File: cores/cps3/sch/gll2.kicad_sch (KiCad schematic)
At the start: 1 part

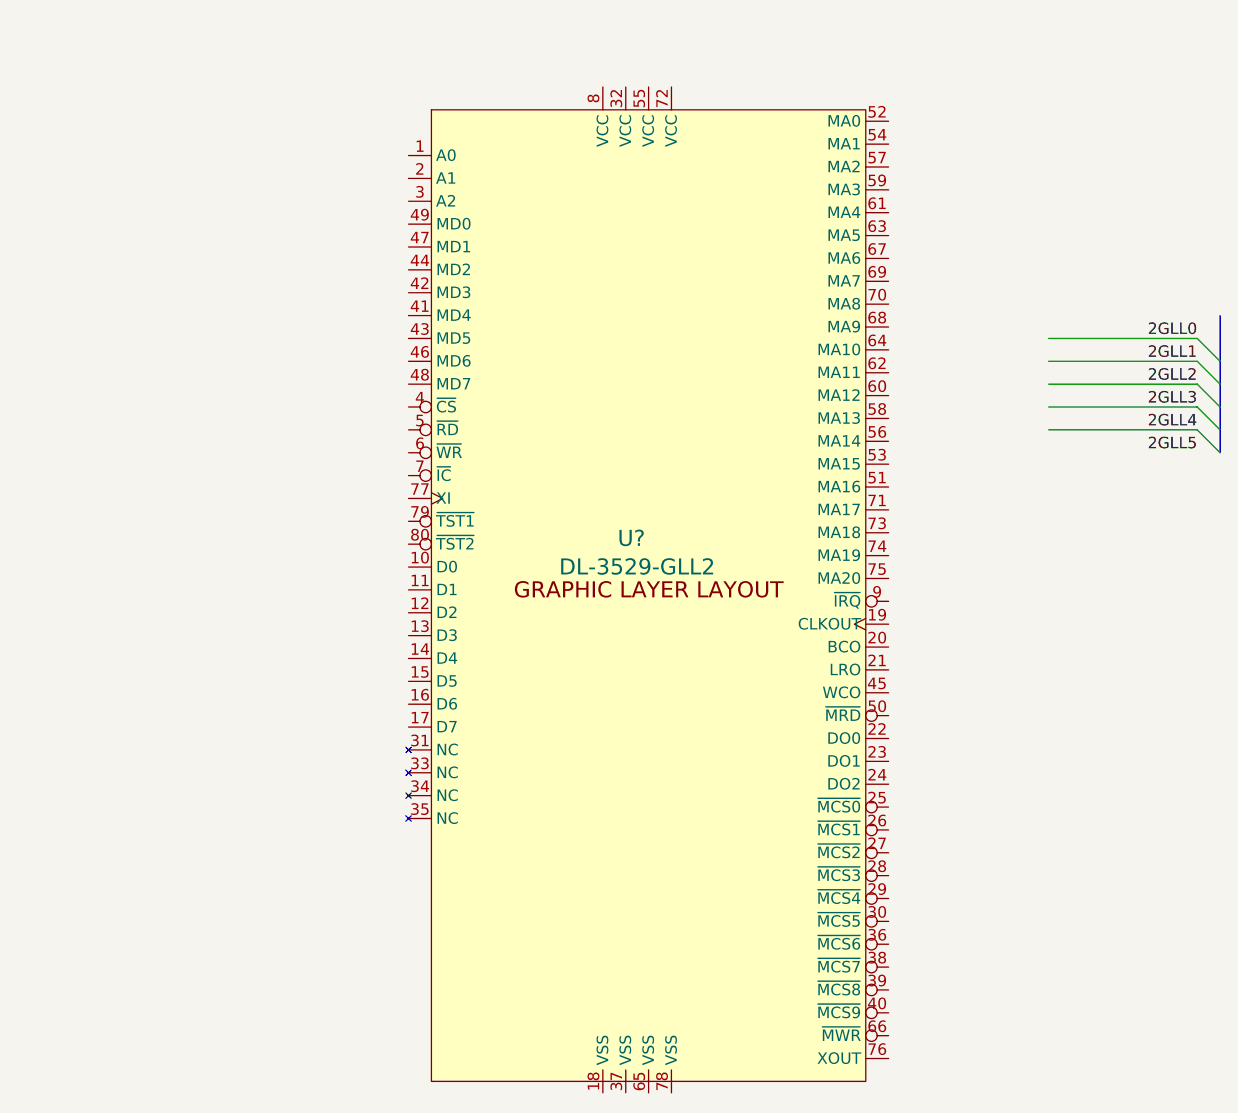
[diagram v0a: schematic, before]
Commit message: iou
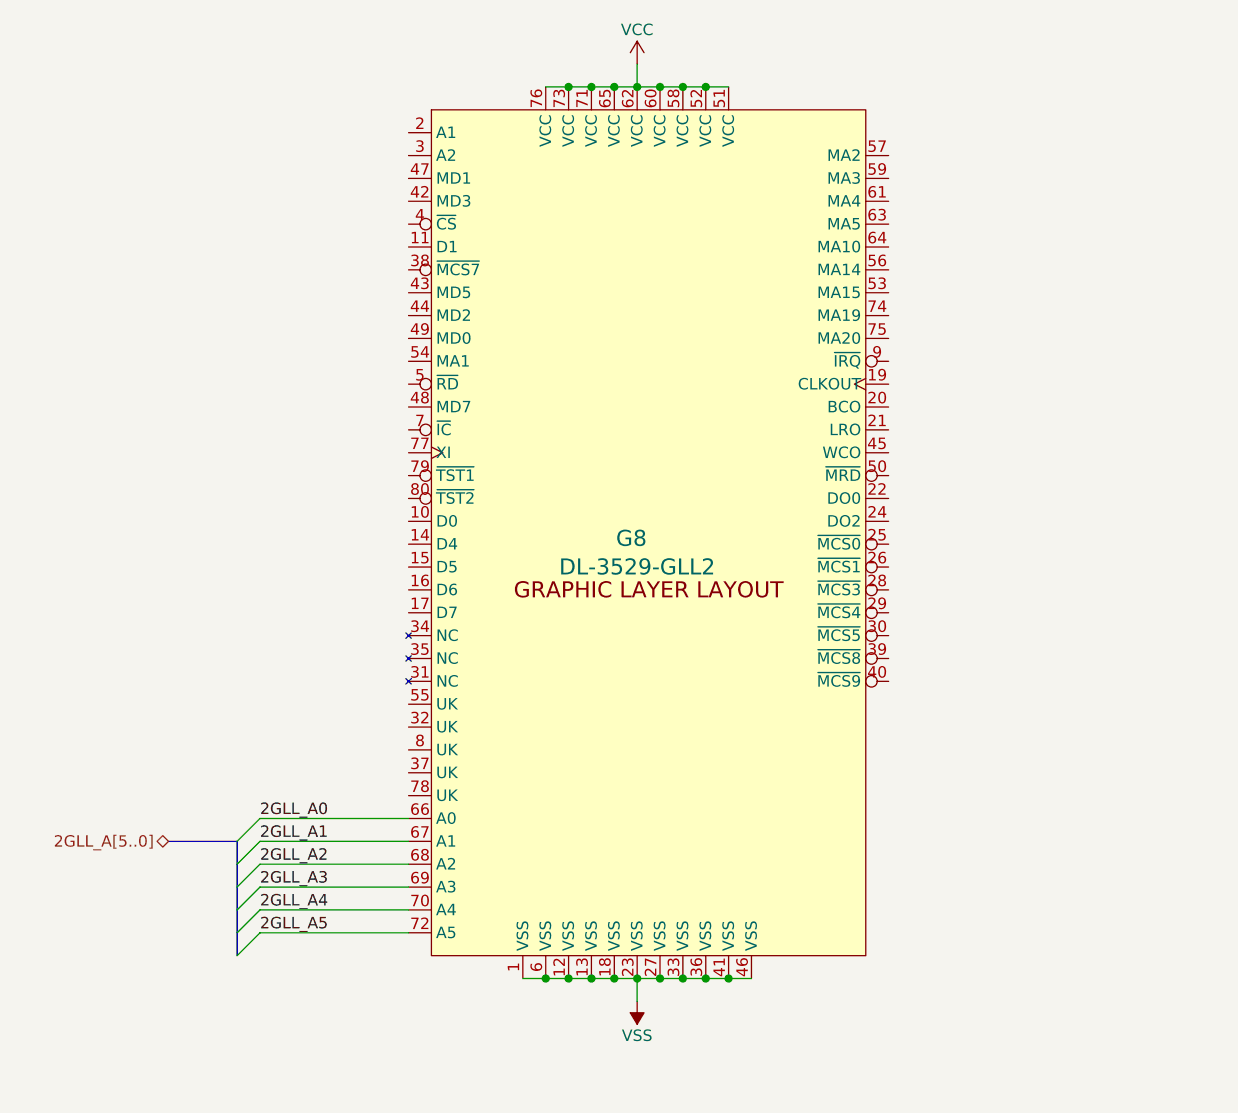
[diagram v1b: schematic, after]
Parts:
- gave numbers to parts that had none: 1
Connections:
- net VSS: now reaches G8.1 (VSS)
- net VSS: now also G8.12 (VSS), G8.13 (VSS), G8.18 (VSS), G8.23 (VSS), G8.27 (VSS), G8.33 (VSS), G8.36 (VSS), G8.41 (VSS), G8.46 (VSS), G8.6 (VSS)
- net VCC: now reaches G8.51 (VCC)
- net VCC: now also G8.52 (VCC), G8.58 (VCC), G8.60 (VCC), G8.62 (VCC), G8.65 (VCC), G8.71 (VCC), G8.73 (VCC), G8.76 (VCC)
- net 2GLL_A0: now reaches G8.66 (A0)
- net 2GLL_A1: now reaches G8.67 (A1)
- net 2GLL_A2: now reaches G8.68 (A2)
- net 2GLL_A3: now reaches G8.69 (A3)
- net 2GLL_A4: now reaches G8.70 (A4)
- net 2GLL_A5: now reaches G8.72 (A5)
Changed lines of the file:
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@@
     (comment 1 "E.Triana")
   )
-  (bus_entry (at 184.15 72.39) (size 2.54 2.54)
-    (stroke (width 0) (type default) (color 0 0 0 0))
-  )
-  (bus_entry (at 184.15 69.85) (size 2.54 2.54)
-    (stroke (width 0) (type default) (color 0 0 0 0))
-  )
-  (bus_entry (at 184.15 67.31) (size 2.54 2.54)
-    (stroke (width 0) (type default) (color 0 0 0 0))
-  )
-  (bus_entry (at 184.15 64.77) (size 2.54 2.54)
-    (stroke (width 0) (type default) (color 0 0 0 0))
-  )
-  (bus_entry (at 184.15 62.23) (size 2.54 2.54)
-    (stroke (width 0) (type default) (color 0 0 0 0))
-  )
-  (bus (pts (xy 186.69 72.39) (xy 186.69 74.93))
-    (stroke (width 0) (type default) (color 0 0 0 0))
-  )
-  (wire (pts (xy 184.15 62.23) (xy 167.64 62.23))
-    (stroke (width 0) (type default) (color 0 0 0 0))
-  )
-  (bus (pts (xy 186.69 69.85) (xy 186.69 72.39))
-    (stroke (width 0) (type default) (color 0 0 0 0))
-  )
-  (wire (pts (xy 184.15 69.85) (xy 167.64 69.85))
-    (stroke (width 0) (type default) (color 0 0 0 0))
-  )
-  (wire (pts (xy 184.15 67.31) (xy 167.64 67.31))
-    (stroke (width 0) (type default) (color 0 0 0 0))
-  )
-  (bus (pts (xy 186.69 67.31) (xy 186.69 69.85))
-    (stroke (width 0) (type default) (color 0 0 0 0))
-  )
-  (bus (pts (xy 186.69 59.69) (xy 186.69 64.77))
-    (stroke (width 0) (type default) (color 0 0 0 0))
-  )
-  (bus (pts (xy 186.69 64.77) (xy 186.69 67.31))
-    (stroke (width 0) (type default) (color 0 0 0 0))
-  )
-  (wire (pts (xy 184.15 64.77) (xy 167.64 64.77))
-    (stroke (width 0) (type default) (color 0 0 0 0))
-  )
-  (wire (pts (xy 184.15 72.39) (xy 167.64 72.39))
+  (junction (at 124.46 34.29) (diameter 0) (color 0 0 0 0)
+  )
+  (junction (at 119.38 133.35) (diameter 0) (color 0 0 0 0)
+  )
+  (junction (at 116.84 34.29) (diameter 0) (color 0 0 0 0)
+  )
+  (junction (at 129.54 133.35) (diameter 0) (color 0 0 0 0)
+  )
+  (junction (at 116.84 133.35) (diameter 0) (color 0 0 0 0)
+  )
+  (junction (at 132.08 133.35) (diameter 0) (color 0 0 0 0)
+  )
+  (junction (at 121.92 133.35) (diameter 0) (color 0 0 0 0)
+  )
+  (junction (at 124.46 133.35) (diameter 0) (color 0 0 0 0)
+  )
+  (junction (at 127 34.29) (diameter 0) (color 0 0 0 0)
+  )
+  (junction (at 127 133.35) (diameter 0) (color 0 0 0 0)
+  )
+  (junction (at 121.92 34.29) (diameter 0) (color 0 0 0 0)
+  )
+  (junction (at 111.76 133.35) (diameter 0) (color 0 0 0 0)
+  )
+  (junction (at 119.38 34.29) (diameter 0) (color 0 0 0 0)
+  )
+  (junction (at 129.54 34.29) (diameter 0) (color 0 0 0 0)
+  )
+  (junction (at 114.3 34.29) (diameter 0) (color 0 0 0 0)
+  )
+  (junction (at 114.3 133.35) (diameter 0) (color 0 0 0 0)
+  )
+  (bus_entry (at 80.01 125.73) (size -2.54 2.54)
+    (stroke (width 0) (type default) (color 0 0 0 0))
+  )
+  (bus_entry (at 80.01 123.19) (size -2.54 2.54)
+    (stroke (width 0) (type default) (color 0 0 0 0))
+  )
+  (bus_entry (at 80.01 120.65) (size -2.54 2.54)
+    (stroke (width 0) (type default) (color 0 0 0 0))
+  )
+  (bus_entry (at 80.01 118.11) (size -2.54 2.54)
+    (stroke (width 0) (type default) (color 0 0 0 0))
+  )
+  (bus_entry (at 80.01 115.57) (size -2.54 2.54)
+    (stroke (width 0) (type default) (color 0 0 0 0))
+  )
+  (bus_entry (at 77.47 130.81) (size 2.54 -2.54)
+    (stroke (width 0) (type default) (color 0 0 0 0))
+  )
+  (wire (pts (xy 116.84 34.29) (xy 119.38 34.29))
+    (stroke (width 0) (type default) (color 0 0 0 0))
+  )
+  (wire (pts (xy 80.01 128.27) (xy 96.52 128.27))
+    (stroke (width 0) (type default) (color 0 0 0 0))
+  )
+  (bus (pts (xy 77.47 125.73) (xy 77.47 128.27))
+    (stroke (width 0) (type default) (color 0 0 0 0))
+  )
+  (wire (pts (xy 80.01 115.57) (xy 96.52 115.57))
+    (stroke (width 0) (type default) (color 0 0 0 0))
+  )
+  (wire (pts (xy 114.3 133.35) (xy 116.84 133.35))
+    (stroke (width 0) (type default) (color 0 0 0 0))
+  )
+  (wire (pts (xy 127 34.29) (xy 129.54 34.29))
+    (stroke (width 0) (type default) (color 0 0 0 0))
+  )
+  (bus (pts (xy 77.47 123.19) (xy 77.47 125.73))
+    (stroke (width 0) (type default) (color 0 0 0 0))
+  )
+  (wire (pts (xy 121.92 34.29) (xy 124.46 34.29))
+    (stroke (width 0) (type default) (color 0 0 0 0))
+  )
+  (wire (pts (xy 114.3 34.29) (xy 116.84 34.29))
+    (stroke (width 0) (type default) (color 0 0 0 0))
+  )
+  (wire (pts (xy 121.92 31.75) (xy 121.92 34.29))
+    (stroke (width 0) (type default) (color 0 0 0 0))
+  )
+  (wire (pts (xy 121.92 133.35) (xy 121.92 135.89))
+    (stroke (width 0) (type default) (color 0 0 0 0))
+  )
+  (wire (pts (xy 129.54 133.35) (xy 132.08 133.35))
+    (stroke (width 0) (type default) (color 0 0 0 0))
+  )
+  (wire (pts (xy 80.01 123.19) (xy 96.52 123.19))
+    (stroke (width 0) (type default) (color 0 0 0 0))
+  )
+  (wire (pts (xy 132.08 133.35) (xy 134.62 133.35))
+    (stroke (width 0) (type default) (color 0 0 0 0))
+  )
+  (wire (pts (xy 80.01 120.65) (xy 96.52 120.65))
+    (stroke (width 0) (type default) (color 0 0 0 0))
+  )
+  (wire (pts (xy 119.38 34.29) (xy 121.92 34.29))
+    (stroke (width 0) (type default) (color 0 0 0 0))
+  )
+  (bus (pts (xy 77.47 120.65) (xy 77.47 123.19))
+    (stroke (width 0) (type default) (color 0 0 0 0))
+  )
+  (wire (pts (xy 124.46 34.29) (xy 127 34.29))
+    (stroke (width 0) (type default) (color 0 0 0 0))
+  )
+  (bus (pts (xy 69.85 118.11) (xy 77.47 118.11))
+    (stroke (width 0) (type default) (color 0 0 0 0))
+  )
+  (bus (pts (xy 77.47 118.11) (xy 77.47 120.65))
+    (stroke (width 0) (type default) (color 0 0 0 0))
+  )
+  (wire (pts (xy 124.46 133.35) (xy 127 133.35))
+    (stroke (width 0) (type default) (color 0 0 0 0))
+  )
+  (wire (pts (xy 127 133.35) (xy 129.54 133.35))
+    (stroke (width 0) (type default) (color 0 0 0 0))
+  )
+  (wire (pts (xy 129.54 34.29) (xy 132.08 34.29))
+    (stroke (width 0) (type default) (color 0 0 0 0))
+  )
+  (bus (pts (xy 77.47 128.27) (xy 77.47 130.81))
+    (stroke (width 0) (type default) (color 0 0 0 0))
+  )
+  (wire (pts (xy 109.22 133.35) (xy 111.76 133.35))
+    (stroke (width 0) (type default) (color 0 0 0 0))
+  )
+  (wire (pts (xy 111.76 133.35) (xy 114.3 133.35))
+    (stroke (width 0) (type default) (color 0 0 0 0))
+  )
+  (wire (pts (xy 119.38 133.35) (xy 121.92 133.35))
+    (stroke (width 0) (type default) (color 0 0 0 0))
+  )
+  (wire (pts (xy 80.01 118.11) (xy 96.52 118.11))
+    (stroke (width 0) (type default) (color 0 0 0 0))
+  )
+  (wire (pts (xy 80.01 125.73) (xy 96.52 125.73))
+    (stroke (width 0) (type default) (color 0 0 0 0))
+  )
+  (wire (pts (xy 111.76 34.29) (xy 114.3 34.29))
+    (stroke (width 0) (type default) (color 0 0 0 0))
+  )
+  (wire (pts (xy 116.84 133.35) (xy 119.38 133.35))
+    (stroke (width 0) (type default) (color 0 0 0 0))
+  )
+  (wire (pts (xy 121.92 133.35) (xy 124.46 133.35))
     (stroke (width 0) (type default) (color 0 0 0 0))
   )
@@
     )
   )
-  (label "2GLL0" (at 184.15 62.23 180)
-    (effects (font (size 1.27 1.27)) (justify right bottom))
-  )
-  (label "2GLL5" (at 184.15 74.93 180)
-    (effects (font (size 1.27 1.27)) (justify right bottom))
-  )
-  (label "2GLL3" (at 184.15 69.85 180)
-    (effects (font (size 1.27 1.27)) (justify right bottom))
-  )
-  (label "2GLL4" (at 184.15 72.39 180)
-    (effects (font (size 1.27 1.27)) (justify right bottom))
-  )
-  (label "2GLL1" (at 184.15 64.77 180)
-    (effects (font (size 1.27 1.27)) (justify right bottom))
-  )
-  (label "2GLL2" (at 184.15 67.31 180)
-    (effects (font (size 1.27 1.27)) (justify right bottom))
+  (label "2GLL_A0" (at 80.01 115.57 0)
+    (effects (font (size 1.27 1.27)) (justify left bottom))
+  )
+  (label "2GLL_A5" (at 80.01 128.27 0)
+    (effects (font (size 1.27 1.27)) (justify left bottom))
+  )
+  (label "2GLL_A3" (at 80.01 123.19 0)
+    (effects (font (size 1.27 1.27)) (justify left bottom))
+  )
+  (label "2GLL_A4" (at 80.01 125.73 0)
+    (effects (font (size 1.27 1.27)) (justify left bottom))
+  )
+  (label "2GLL_A1" (at 80.01 118.11 0)
+    (effects (font (size 1.27 1.27)) (justify left bottom))
+  )
+  (label "2GLL_A2" (at 80.01 120.65 0)
+    (effects (font (size 1.27 1.27)) (justify left bottom))
+  )
+  (hierarchical_label "2GLL_A[5..0]" (shape bidirectional) (at 69.85 118.11 180)
+    (effects (font (size 1.27 1.27)) (justify right))
+  )
+  (symbol (lib_id "power:VSS") (at 121.92 135.89 180) (unit 1)
+    (in_bom yes) (on_board yes)
+    (property "Reference" "#PWR?" (id 0) (at 121.92 132.08 0)
+      (effects (font (size 1.27 1.27)) hide)
+    )
+    (property "Value" "VSS" (id 1) (at 121.92 139.7 0))
+    (property "Footprint" "" (id 2) (at 121.92 135.89 0)
+      (effects (font (size 1.27 1.27)) hide)
+    )
+    (property "Datasheet" "" (id 3) (at 121.92 135.89 0)
+      (effects (font (size 1.27 1.27)) hide)
+    )
+    (pin "1")
   )
   (symbol (lib_id "capcom:DL-3529-GLL2") (at 121.92 87.63 0) (unit 1)
     (in_bom yes) (on_board yes)
-    (property "Reference" "U?" (id 0) (at 121.285 84.455 0)
+    (property "Reference" "G8" (id 0) (at 121.285 84.455 0)
       (effects (font (size 1.778 1.778)))
     )
@@
     (pin "9")
   )
+  (symbol (lib_id "power:VCC") (at 121.92 31.75 0) (unit 1)
+    (in_bom yes) (on_board yes)
+    (property "Reference" "#PWR?" (id 0) (at 121.92 35.56 0)
+      (effects (font (size 1.27 1.27)) hide)
+    )
+    (property "Value" "VCC" (id 1) (at 121.92 27.94 0))
+    (property "Footprint" "" (id 2) (at 121.92 31.75 0)
+      (effects (font (size 1.27 1.27)) hide)
+    )
+    (property "Datasheet" "" (id 3) (at 121.92 31.75 0)
+      (effects (font (size 1.27 1.27)) hide)
+    )
+    (pin "1")
+  )
 )
